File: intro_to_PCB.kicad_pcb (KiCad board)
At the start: 2 copper layers, 0 parts

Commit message: final intro pcb
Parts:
- added C1: .1u, Capacitor_SMD:C_0402_1005Metric_Pad0.74x0.62mm_HandSolder, F.Cu at (193.5, 52.1)
- added C10: .1u, Capacitor_SMD:C_0603_1608Metric_Pad1.08x0.95mm_HandSolder, F.Cu at (144.6, 70.5)
- added C11: 4.7u, Capacitor_SMD:C_Elec_6.3x7.7, F.Cu at (140.5, 77.0)
- added C12: .1u, Capacitor_SMD:C_0402_1005Metric_Pad0.74x0.62mm_HandSolder, F.Cu at (153.5, 66.0)
- added C13: C, Capacitor_SMD:C_0603_1608Metric_Pad1.08x0.95mm_HandSolder, F.Cu at (153.1, 67.5)
- added C14: 4.7u, Capacitor_SMD:C_Elec_6.3x7.7, F.Cu at (152.5, 42.5)
- added C15: .1u, Capacitor_SMD:C_Elec_6.3x7.7, F.Cu at (161.5, 42.5)
- added C2: .1u, Capacitor_SMD:C_0402_1005Metric_Pad0.74x0.62mm_HandSolder, F.Cu at (199.9, 51.5)
- added C3: .1u, Capacitor_SMD:C_0603_1608Metric_Pad1.08x0.95mm_HandSolder, F.Cu at (194.0, 67.1)
- added C4: .1u, Capacitor_SMD:C_0603_1608Metric_Pad1.08x0.95mm_HandSolder, F.Cu at (192.0, 67.1)
- added C5: 18p, Capacitor_SMD:C_0402_1005Metric_Pad0.74x0.62mm_HandSolder, F.Cu at (195.0, 70.5)
- added C6: 18p, Capacitor_SMD:C_0402_1005Metric_Pad0.74x0.62mm_HandSolder, F.Cu at (199.0, 70.5)
- added C7: 10u, Capacitor_SMD:C_Elec_6.3x7.7, F.Cu at (149.0, 77.0)
- added C8: .1u, Capacitor_SMD:C_Elec_6.3x7.7, F.Cu at (166.5, 78.5)
- added C9: .01u, Capacitor_SMD:C_0603_1608Metric_Pad1.08x0.95mm_HandSolder, F.Cu at (139.5, 67.5)
- added D1: ESD9B5.0ST5G, Diode_SMD:D_0402_1005Metric_Pad0.77x0.64mm_HandSolder, F.Cu at (146.4, 61.5)
- added D2: ESD9B5.0ST5G, Diode_SMD:D_0402_1005Metric_Pad0.77x0.64mm_HandSolder, F.Cu at (146.3, 62.5)
- added D3: LED, Diode_SMD:D_0402_1005Metric_Pad0.77x0.64mm_HandSolder, F.Cu at (139.6, 52.5)
- added D4: LED, Diode_SMD:D_0402_1005Metric_Pad0.77x0.64mm_HandSolder, F.Cu at (139.5, 50.0)
- added D5: LED, Diode_SMD:D_0402_1005Metric_Pad0.77x0.64mm_HandSolder, F.Cu at (159.5, 66.5)
- added D6: LED, Diode_SMD:D_0402_1005Metric_Pad0.77x0.64mm_HandSolder, F.Cu at (158.0, 66.5)
- added F1: 500mA, Inductor_SMD:L_1812_4532Metric_Pad1.30x3.40mm_HandSolder, F.Cu at (144.5, 83.5)
- added FB1: 120, Fuse:Fuse_0603_1608Metric_Pad1.05x0.95mm_HandSolder, F.Cu at (143.5, 67.5)
- added J1: USB_C_Receptacle_USB2.0_16P, Connector_USB:USB_C_Receptacle_Palconn_UTC16-G, F.Cu at (139.7, 60.5)
- added J2: Conn_01x16_Socket, Connector_PinHeader_2.54mm:PinHeader_1x16_P2.54mm_Vertical, F.Cu at (211.3, 38.0)
- added J3: Conn_01x16_Socket, Connector_PinHeader_2.54mm:PinHeader_1x16_P2.54mm_Vertical, F.Cu at (211.2, 84.5)
- added J4: Conn_PIC_ICSP_ICD, Connector_PinHeader_2.54mm:PinHeader_2x03_P2.54mm_Vertical, F.Cu at (211.5, 62.5)
- added L1: 10u, Inductor_SMD:L_0603_1608Metric_Pad1.05x0.95mm_HandSolder, F.Cu at (196.6, 51.5)
- added R1: 10k, Resistor_SMD:R_0402_1005Metric_Pad0.72x0.64mm_HandSolder, F.Cu at (184.5, 59.5)
- added R10: 70, Resistor_SMD:R_0402_1005Metric_Pad0.72x0.64mm_HandSolder, F.Cu at (142.9, 50.0)
- added R11: R, Resistor_SMD:R_0402_1005Metric_Pad0.72x0.64mm_HandSolder, F.Cu at (159.5, 68.9)
- added R12: R, Resistor_SMD:R_0402_1005Metric_Pad0.72x0.64mm_HandSolder, F.Cu at (158.0, 69.1)
- added R2: 1M, Resistor_SMD:R_0402_1005Metric_Pad0.72x0.64mm_HandSolder, F.Cu at (196.9, 69.9)
- added R3: 4.7k, Resistor_SMD:R_0402_1005Metric_Pad0.72x0.64mm_HandSolder, F.Cu at (186.0, 56.5)
- added R4: 4.7k, Resistor_SMD:R_0402_1005Metric_Pad0.72x0.64mm_HandSolder, F.Cu at (184.0, 56.4)
- added R5: 200, Resistor_SMD:R_0402_1005Metric_Pad0.72x0.64mm_HandSolder, F.Cu at (163.0, 74.0)
- added R6: 121, Resistor_SMD:R_0402_1005Metric_Pad0.72x0.64mm_HandSolder, F.Cu at (160.4, 74.5)
- added R7: 5.1k, Resistor_SMD:R_0402_1005Metric_Pad0.72x0.64mm_HandSolder, F.Cu at (144.5, 59.0)
- added R8: 5.1k, Resistor_SMD:R_0402_1005Metric_Pad0.72x0.64mm_HandSolder, F.Cu at (146.4, 63.5)
- added R9: 155, Resistor_SMD:R_0402_1005Metric_Pad0.72x0.64mm_HandSolder, F.Cu at (143.1, 52.5)
- added SW1: SW_Push, Button_Switch_SMD:SW_Push_SPST_NO_Alps_SKRK, F.Cu at (183.5, 65.0)
- added U1: ATmega328P-A, Package_QFP:TQFP-32_7x7mm_P0.8mm, F.Cu at (193.0, 60.0)
- added U2: LM1117T-ADJ, Package_TO_SOT_SMD:SOT-223, F.Cu at (159.0, 80.0)
- added U3: FT232RL, Package_SO:SSOP-28_5.3x10.2mm_P0.65mm, F.Cu at (158.1, 60.5)
- added Y1: 16MHz, Crystal:Crystal_SMD_2012-2Pin_2.0x1.2mm_HandSoldering, F.Cu at (197.0, 67.4)
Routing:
- net +5V: track 0.00 -> 149.5 mm, vias 0 -> 13
- net GND: track 0.00 -> 116.5 mm, vias 0 -> 45
- net EX_RST: track 0.00 -> 113.5 mm, vias 0 -> 4
- net +3.3V: track 0.00 -> 113.0 mm, vias 0 -> 2
- net PWRU_IN: track 0.00 -> 108.4 mm, vias 0 -> 1
- net USART_RXD: track 0.00 -> 58.0 mm, vias 0 -> 2
- net USART_TXD: track 0.00 -> 56.8 mm
- net SPI_SCK: track 0.00 -> 55.7 mm, vias 0 -> 1
- net SPI_MISO: track 0.00 -> 42.9 mm, vias 0 -> 1
- net SPI_MOSI: track 0.00 -> 41.5 mm, vias 0 -> 1
- net SPI_SS: track 0.00 -> 38.2 mm
- net GPIO_D5: track 0.00 -> 38.0 mm
- net GPIO_D6: track 0.00 -> 36.8 mm
- net GPIO_C5: track 0.00 -> 36.2 mm, vias 0 -> 1
- net GPIO_D7: track 0.00 -> 35.9 mm
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- added copper zone on B.Cu, net +5V
- added copper zone on B.Cu, net GND
- added copper zone on F.Cu, net GND
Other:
- board outline added: 78 x 50.5 mm
- board text added: "+3.3V"
- board text added: "+5.0V"
- board text added: "Alex Forrest SoCET"
- board text added: "EX_IN"
- board text added: "GND"
- board text added: "IO_B0"
- board text added: "IO_B1"
- board text added: "IO_C0"
- board text added: "IO_C1"
- board text added: "IO_C2"
- board text added: "IO_C3"
- board text added: "IO_C4"
- board text added: "IO_C5"
- board text added: "IO_D2"
- board text added: "IO_D3"
- board text added: "IO_D4"
- board text added: "IO_D5"
- board text added: "IO_D6"
- board text added: "IO_D7"
- board text added: "MISO"
- board text added: "MOSI"
- board text added: "RST"
- board text added: "RX"
- board text added: "SCK"
- board text added: "SCL"
- board text added: "SDA"
- board text added: "SS"
- board text added: "TX"

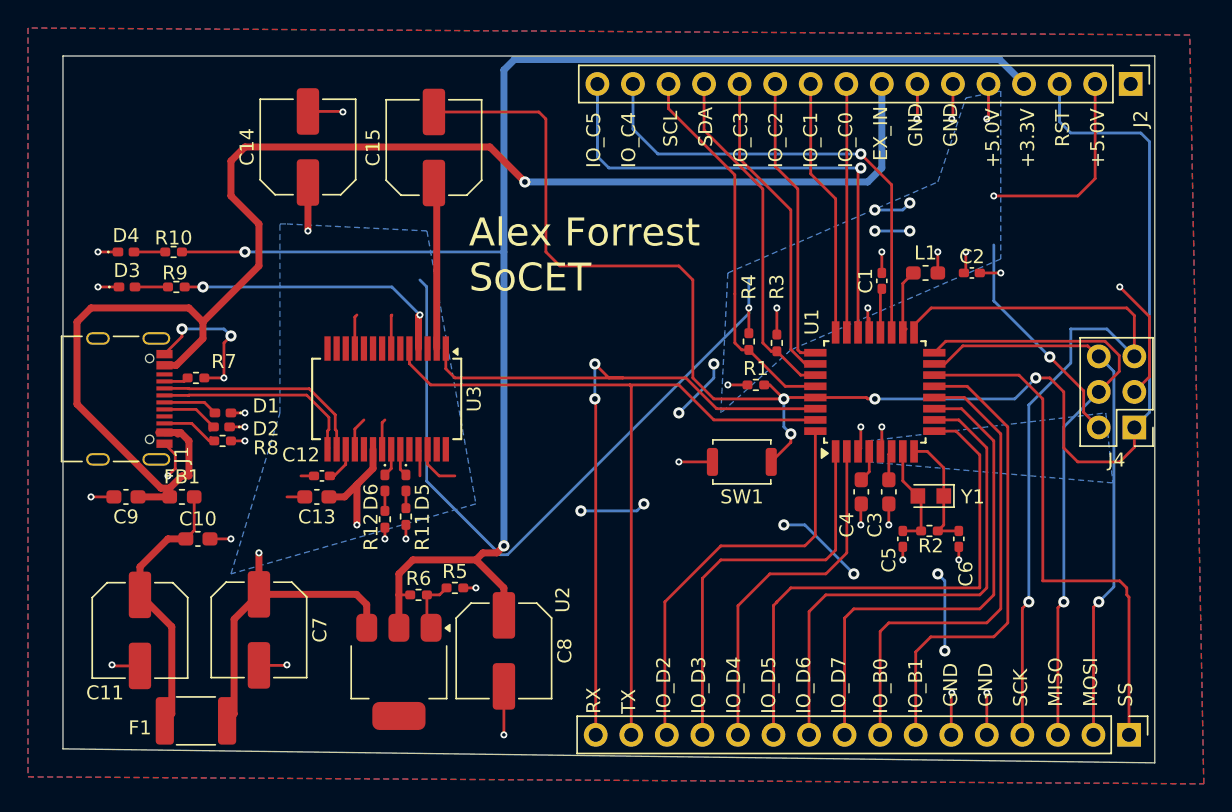
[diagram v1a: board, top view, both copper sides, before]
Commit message: fixed clearance
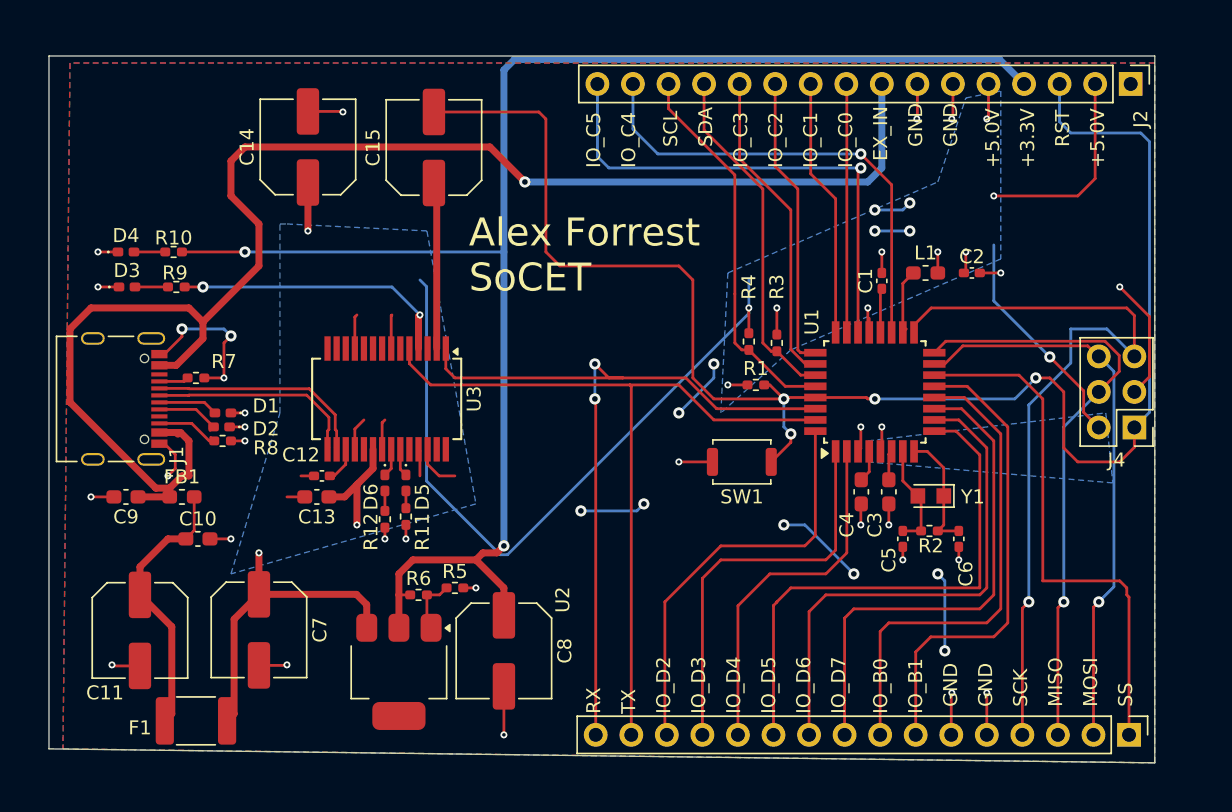
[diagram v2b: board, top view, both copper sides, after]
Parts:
- moved J1 0.37 mm to (139.4, 60.5)
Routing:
- net PWRU_IN: track 108.4 -> 109.1 mm
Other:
- board size 78 x 50.5 mm -> 79 x 50.5 mm
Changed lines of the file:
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@@
 		)
 		(property "Value" "ESD9B5.0ST5G"
-			(at -70.73 -21.79 360)
+			(at -70.73 -21.79 0)
 			(layer "F.Fab")
 			(hide yes)
@@
 		)
 		(fp_text user "${REFERENCE}"
-			(at 0 0 360)
+			(at 0 0 0)
 			(layer "F.Fab")
 			(effects
@@
 		(tags "resistor handsolder")
 		(property "Reference" "R10"
-			(at 0 1 360)
+			(at 0 1 0)
 			(layer "F.SilkS")
 			(effects
@@
 		)
 		(property "Value" "70"
-			(at 0 1.17 360)
+			(at 0 1.17 0)
 			(layer "F.Fab")
 			(effects
@@
 		)
 		(fp_text user "${REFERENCE}"
-			(at 0 0 360)
+			(at 0 0 0)
 			(layer "F.Fab")
 			(effects
@@
 		(tags "resistor handsolder")
 		(property "Reference" "R9"
-			(at 0.0975 1 360)
+			(at 0.0975 1 0)
 			(layer "F.SilkS")
 			(effects
@@
 		)
 		(property "Value" "155"
-			(at -74.3275 -38.62 360)
+			(at -74.3275 -38.62 0)
 			(layer "F.Fab")
 			(effects
@@
 		)
 		(fp_text user "${REFERENCE}"
-			(at 0 0 360)
+			(at 0 0 0)
 			(layer "F.Fab")
 			(effects
@@
 	(footprint "Connector_USB:USB_C_Receptacle_Palconn_UTC16-G"
 		(layer "F.Cu")
-		(at 139.74 60.5 -90)
+		(at 139.375 60.5 -90)
 		(descr "http://www.palpilot.com/wp-content/uploads/2017/05/UTC027-GKN-OR-Rev-A.pdf")
 		(tags "USB C Type-C Receptacle USB2.0")
@@
 		(tags "diode handsolder")
 		(property "Reference" "D2"
-			(at -3.17 -0.14 360)
+			(at -3.17 -0.14 0)
 			(layer "F.SilkS")
 			(effects
@@
 		)
 		(property "Value" "ESD9B5.0ST5G"
-			(at -72.6325 -25.29 360)
+			(at -72.6325 -25.29 0)
 			(layer "F.Fab")
 			(effects
@@
 		)
 		(fp_text user "${REFERENCE}"
-			(at 0 0 360)
+			(at 0 0 0)
 			(layer "F.Fab")
 			(effects
@@
 		(tags "SMD SMT button")
 		(property "Reference" "SW1"
-			(at 0 -2.5 360)
+			(at 0 -2.5 0)
 			(layer "F.SilkS")
 			(effects
@@
 		)
 		(fp_text user "${REFERENCE}"
-			(at 0 0 360)
+			(at 0 0 0)
 			(layer "F.Fab")
 			(effects
@@
 	(gr_poly
 		(pts
-			(xy 213 36) (xy 213 86.5) (xy 135 85.5) (xy 135 36)
+			(xy 213 36) (xy 213 86.5) (xy 134 85.5) (xy 134 36)
 		)
 		(stroke
@@
 	)
 	(segment
-		(start 145 55)
-		(end 144 54)
-		(width 0.5)
-		(layer "F.Cu")
-		(net 7)
-	)
-	(segment
-		(start 142.001203 66.875)
-		(end 142.625 66.875)
-		(width 0.5)
-		(layer "F.Cu")
-		(net 7)
-	)
-	(segment
 		(start 142.25 58.1)
 		(end 143.09 58.1)
@@
 	)
 	(segment
-		(start 144 54)
-		(end 137 54)
+		(start 137 54)
+		(end 135.5 55.5)
 		(width 0.5)
 		(layer "F.Cu")
@@
 	)
 	(segment
-		(start 136 55)
-		(end 136 60.873797)
-		(width 0.5)
-		(layer "F.Cu")
-		(net 7)
-	)
-	(segment
 		(start 142.625 66.875)
 		(end 142.625 67.5)
@@
 	)
 	(segment
-		(start 137 54)
-		(end 136 55)
+		(start 144 54)
+		(end 137 54)
 		(width 0.5)
 		(layer "F.Cu")
@@
 	)
 	(segment
+		(start 141.636203 66.875)
+		(end 142.625 66.875)
+		(width 0.5)
+		(layer "F.Cu")
+		(net 7)
+	)
+	(segment
+		(start 145 55)
+		(end 144 54)
+		(width 0.5)
+		(layer "F.Cu")
+		(net 7)
+	)
+	(segment
 		(start 142.25 62.9)
 		(end 143.09 62.9)
@@
 	)
 	(segment
-		(start 136 60.873797)
-		(end 142.001203 66.875)
+		(start 135.5 55.5)
+		(end 135.5 60.738797)
+		(width 0.5)
+		(layer "F.Cu")
+		(net 7)
+	)
+	(segment
+		(start 135.5 60.738797)
+		(end 141.636203 66.875)
 		(width 0.5)
 		(layer "F.Cu")
@@
 		(polygon
 			(pts
-				(xy 132.5 34) (xy 132.5 87.5) (xy 216.5 88) (xy 215.5 34.5)
+				(xy 135.5 36.5) (xy 135 85.5) (xy 213 86.5) (xy 213 36.5)
 			)
 		)
